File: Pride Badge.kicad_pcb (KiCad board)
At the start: 2 copper layers, 93 parts, among them J1 USB_B_Micro, J2 Conn_Batt_JST-PH, J3 SWD_Conn, J4 Conn_SWD20, SW1 PWR_SW, SW2 Mode_BTN, SW3 Bright_BTN, SW4 Reset_BTN, SW5 Boot_SW, SW6 SW_SeeBattGauge, U1 USBLC6-2SC6, U10 555, U2 TP4056, U3 MT3608, U4 AZ1117EH-3.3, U5 FS312F, U6 FS8205, U7 STM32F042F6P6, U8 IS31FL3218, U9 LM339

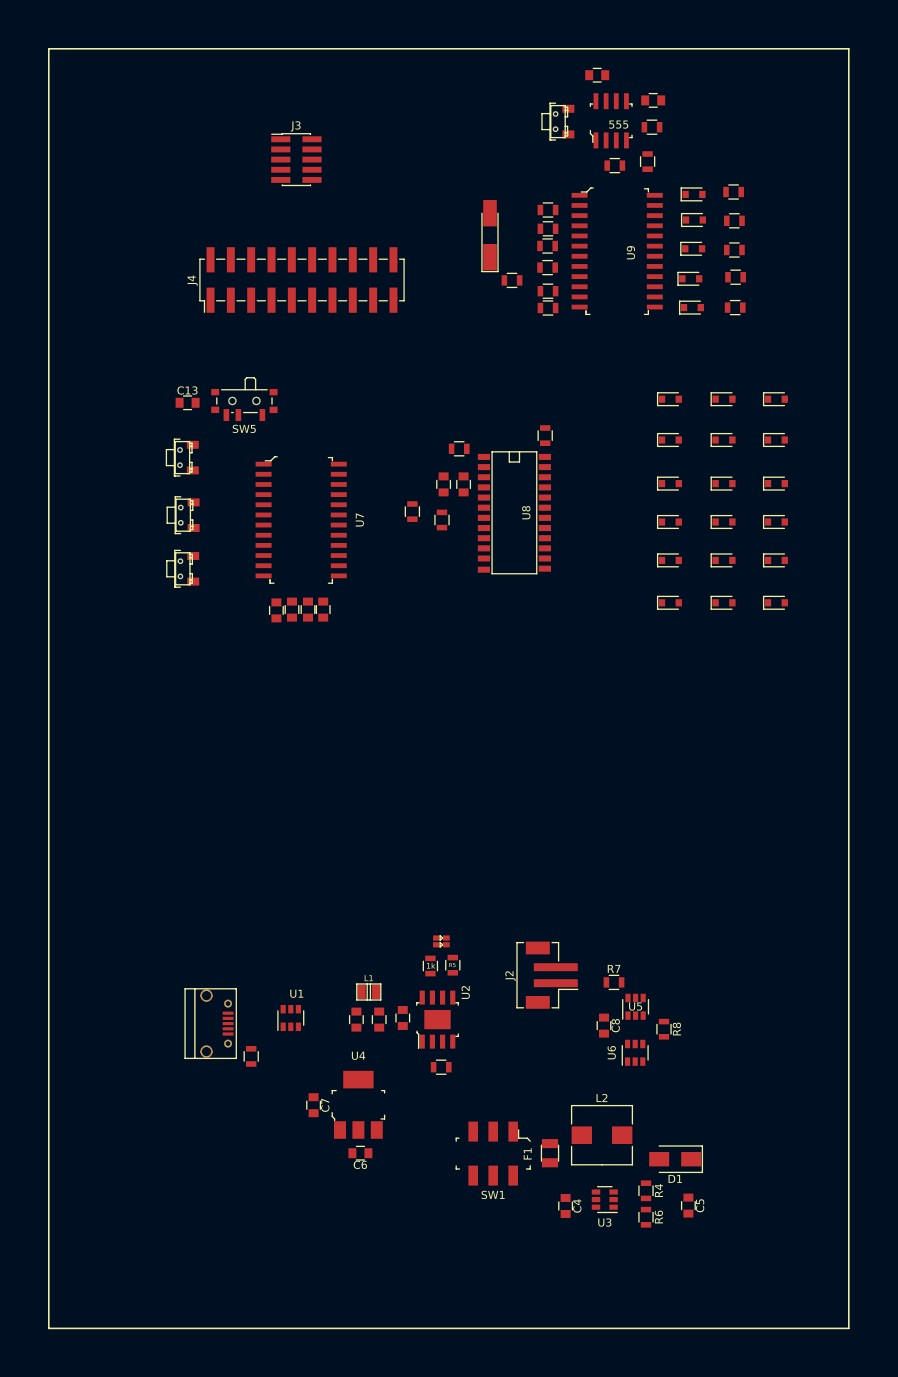
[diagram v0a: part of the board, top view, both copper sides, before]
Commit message: Prototype PCB design finished?
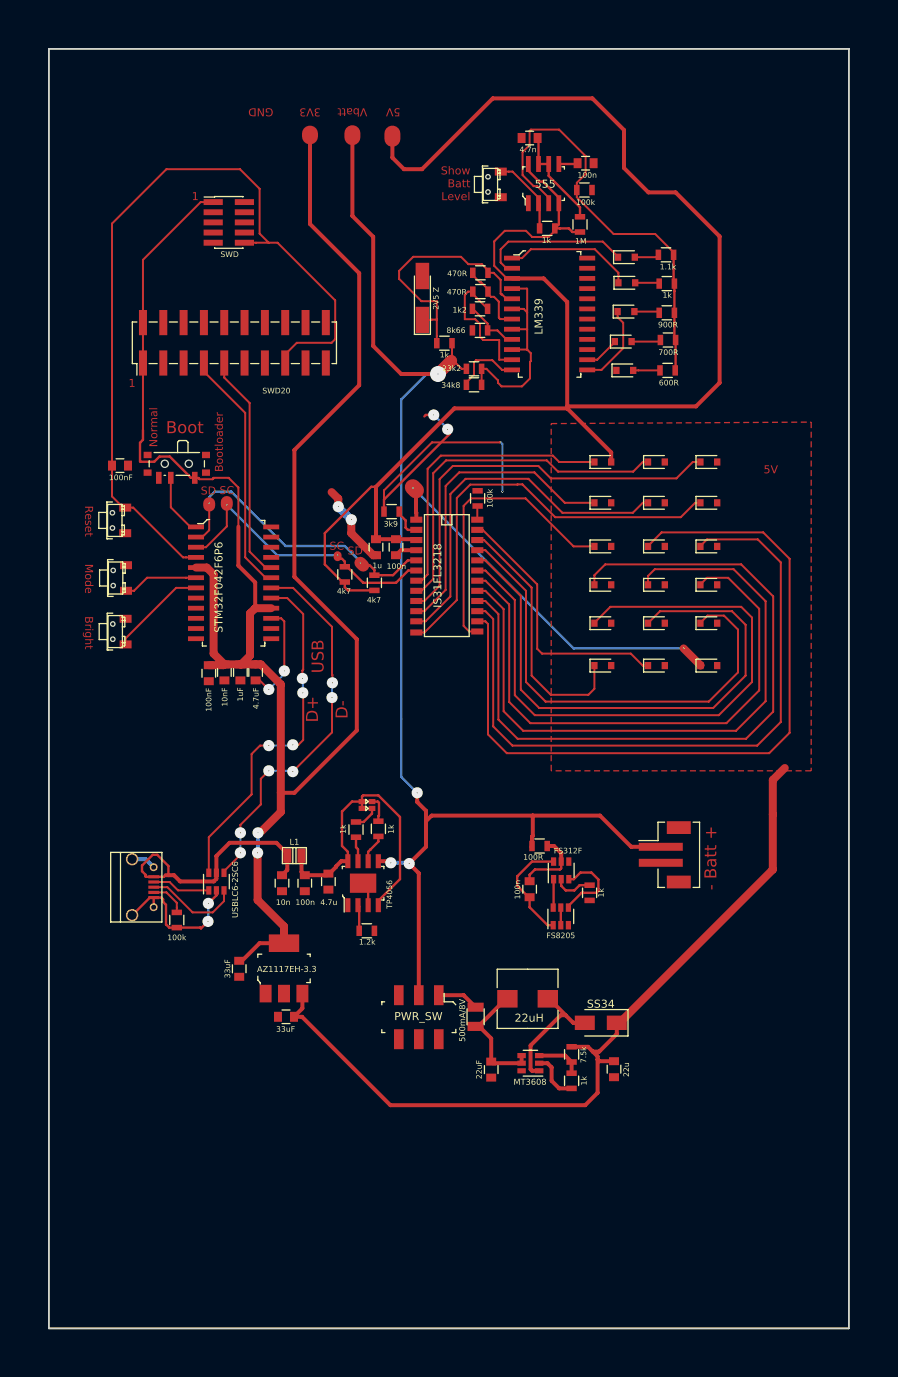
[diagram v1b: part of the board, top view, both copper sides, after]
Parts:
- C14: value 1uF -> 1u
- C15: value 100nF -> 100n
- C4: value 22u -> 22uF
- D3: value 2V5 Zener -> 2V5 Z
- J3: value SWD_Conn -> SWD
- J4: value Conn_SWD20 -> SWD20
- R7: value 100 -> 100R
- moved J2 21.5 mm to (105.3, 117.2), turned to 270 degrees
- moved R2 19.4 mm to (66.1, 114.1)
- moved C3 19.4 mm to (62.6, 120.6)
- moved C6 19.4 mm to (57.4, 137.5)
- moved L1 19.4 mm to (58.4, 117.3)
- moved U1 19.4 mm to (48.6, 120.6)
- moved U4 19.4 mm to (57.1, 131.4)
- moved C4 19.4 mm to (83.0, 144.1)
- moved C7 19.4 mm to (51.5, 131.5)
- moved D1 19.4 mm to (96.7, 138.2)
- moved F1 19.4 mm to (81.0, 137.5)
- moved L2 19.4 mm to (87.5, 135.2)
- moved R3 19.4 mm to (67.5, 126.8)
- moved R4 19.4 mm to (93.0, 142.2)
- moved R5 19.4 mm to (68.9, 114.0)
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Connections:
- D2 pad 1: /SheetPower/VUSB -> Net-(C2-Pad1)
- D2 pad 2: /SheetPower/VUSB -> Net-(C2-Pad1)
- U1 pad 4: (no net) -> USBDM
- U1 pad 6: (no net) -> USBDP
- U7 pad 17: (no net) -> USBDP
- U7 pad 18: (no net) -> USBDM
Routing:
- net +5V: track 0.00 -> 318.8 mm
- net +3V3: track 0.00 -> 241.7 mm, vias 0 -> 2
- net +BATT: track 0.00 -> 166.4 mm, vias 0 -> 4
- net GND: track 0.00 -> 110.5 mm, vias 0 -> 11
- net /Sheet_MCU-LED-Driver/RESET: track 0.00 -> 104.5 mm
- net Net-(DC2-Pad1): track 0.00 -> 96.6 mm
- net Net-(DD1-Pad1): track 0.00 -> 93.4 mm
- net Net-(DC3-Pad1): track 0.00 -> 85.6 mm
- net Net-(DD2-Pad1): track 0.00 -> 82.6 mm
- net Net-(DE1-Pad1): track 0.00 -> 79.7 mm
- net Net-(DD3-Pad1): track 0.00 -> 71.0 mm
- net Net-(DE2-Pad1): track 0.00 -> 69.6 mm
- net Net-(DE3-Pad1): track 0.00 -> 59.8 mm
- net /SheetBatteryGauge/LED_VCC: track 0.00 -> 54.9 mm
- net Net-(DB3-Pad1): track 0.00 -> 53.1 mm
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- added copper zone on F.Cu, net +5V
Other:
- board outline added: 100 x 159.9 mm
- net class Default: clearance 0.2 -> 0.3; via_dia 0.8 -> 2; via_drill 0.4 -> 1
- rule trace_clearance: 0.2 -> 0.3
- rule trace_min: 0.2 -> 0.25
- rule via_min_drill: 0.3 -> 0.1
- rule via_min_size: 0.4 -> 0.2
- board text added: "- Batt +"
- board text added: "1"
- board text added: "3V3"
- board text added: "5V"
- board text added: "Boot"
- board text added: "Bootloader"
- board text added: "Bright"
- board text added: "D+"
- board text added: "D-"
- board text added: "GND"
- board text added: "Mode"
- board text added: "Normal"
- board text added: "Reset"
- board text added: "SC"
- board text added: "SD"
- board text added: "Show Batt Level"
- board text added: "USB"
- board text added: "Vbatt"
